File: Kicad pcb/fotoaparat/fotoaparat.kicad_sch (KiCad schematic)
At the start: 27 parts, among them J1 USB Konektor, J2 SWD, J3 LCD konektor, J5 Sd Karta, J6 UART, J7 Kamera, U1 STM32L496RETx, U2 Regulator 3.3v, U3 MCP73833-FCI/UN, Y1 HC49S-8-30-50-70-30-ATF

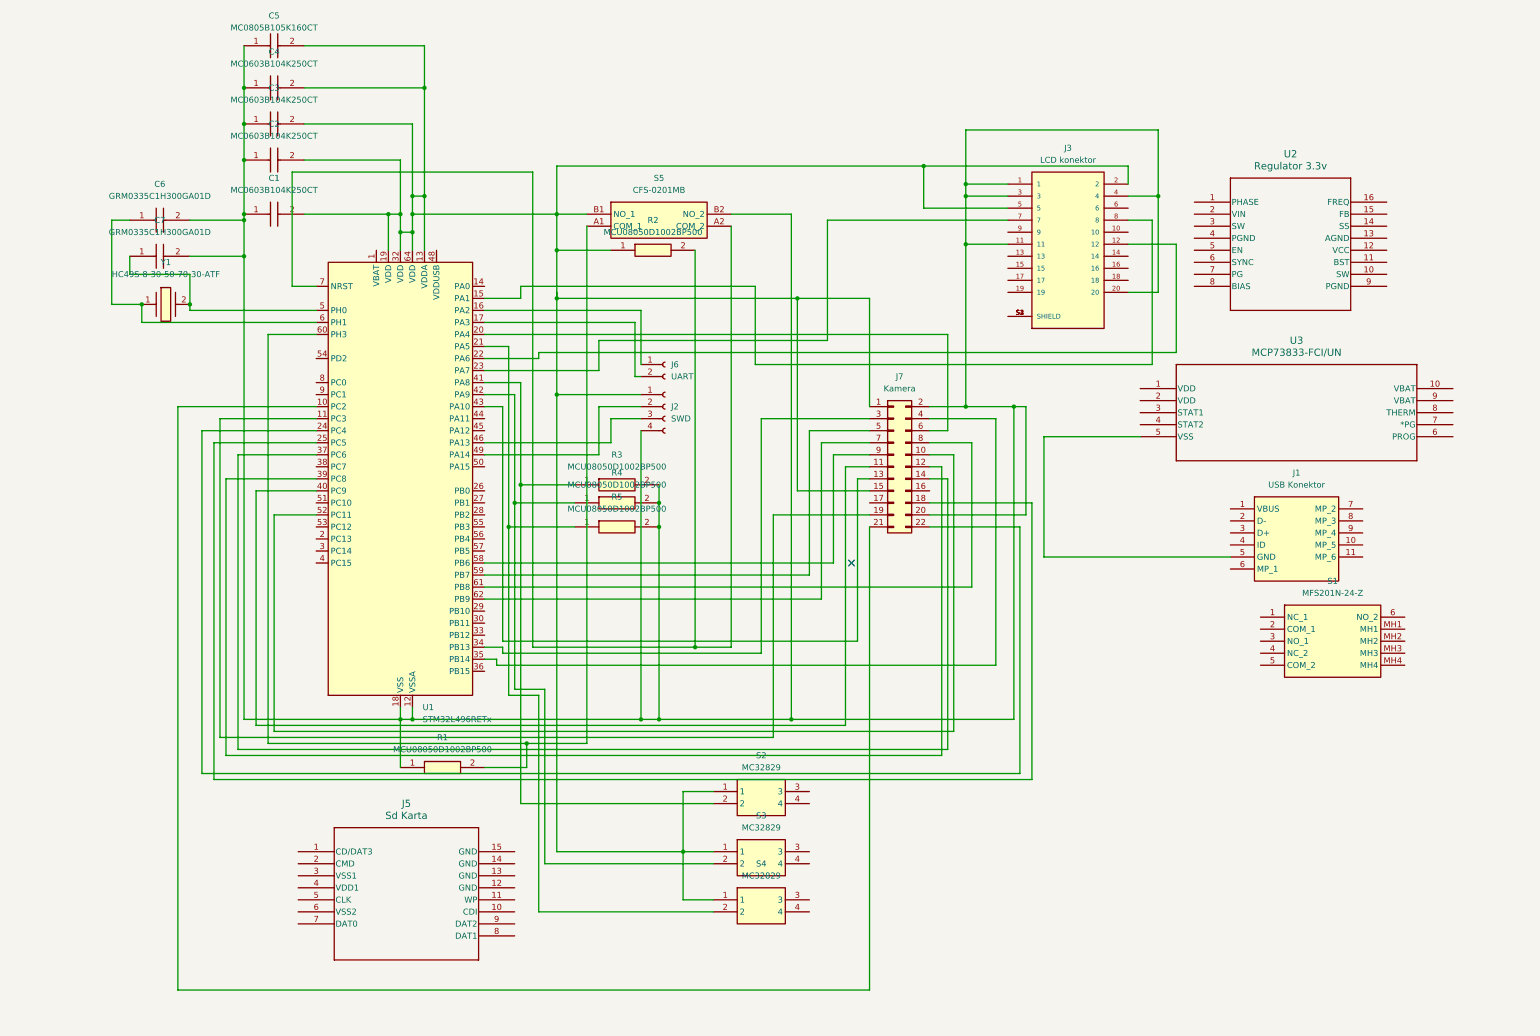
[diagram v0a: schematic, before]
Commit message: Baterie
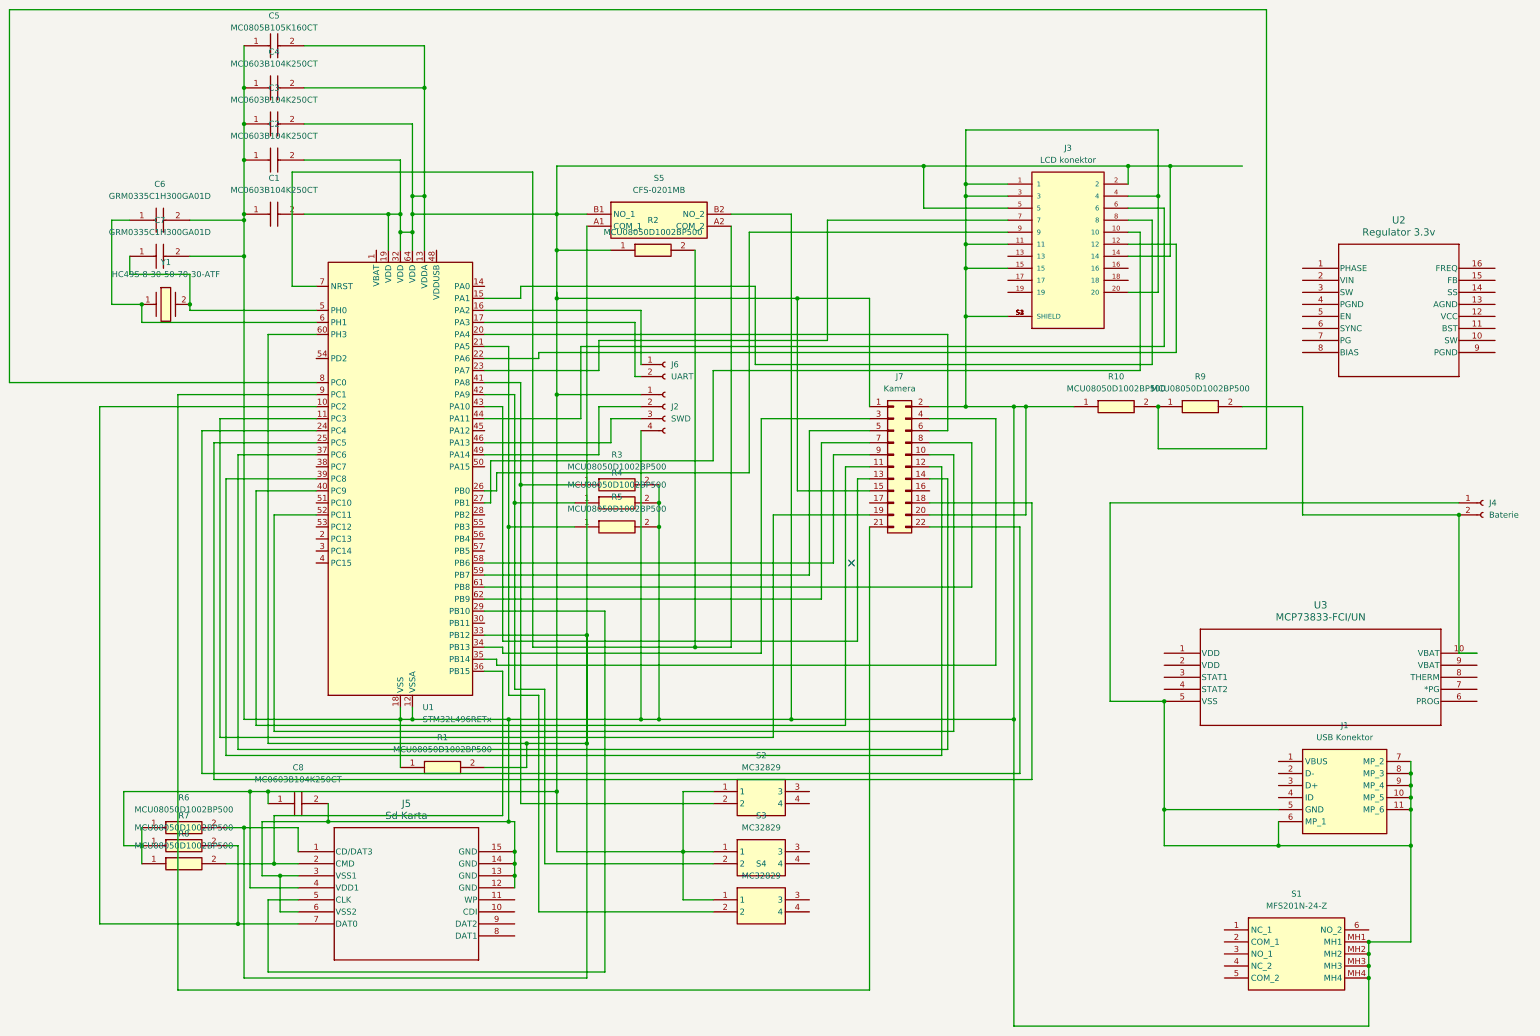
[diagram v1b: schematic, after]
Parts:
- added C8: MC0603B104K250CT, mc06:CAPC1608X87N, symbol MC0603B104K250CT:MC0603B104K250CT
- added J4: Baterie, symbol Connector:Conn_01x02_Socket
- added R10, R6, R7, R8, R9: MCU08050D1002BP500, 2012:RESC2012X55N, symbol MCU08050D1002BP500:MCU08050D1002BP500
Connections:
- net at S1.MH1: now also C1.1, C2.1, C3.1, C4.1, C5.1, C6.2, C7.2, J1.10 (MP_5), J1.11 (MP_6), J1.5 (GND), J1.6 (MP_1), J1.7 (MP_2), J1.8 (MP_3), J1.9 (MP_4), J2.4 (Pin_4), J3.1, J3.11, J3.15, J3.20, J3.3, J3.4, J3.S1 (SHIELD), J3.S2 (SHIELD), J3.S3 (SHIELD), J3.S4 (SHIELD), J5.12 (GND), J5.13 (GND), J5.14 (GND), J5.15 (GND), J5.3 (VSS1), J5.6 (VSS2), J7.2 (Pin_2), J7.20 (Pin_20), R1.1, R3.2, R4.2, R5.2, S1.MH2, S1.MH3, S1.MH4, S5.B2 (NO_2), U1.12 (VSSA), U1.18 (VSS), U1.31 (VSS), U1.47 (VSS), U1.63 (VSS), U3.5 (VSS), C8.2, J4.1 (Pin_1), R10.1
- net at C1.2, C2.2, C3.2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: now also J3.14, J5.4 (VDD1), C8.1, R6.1, R7.1, R8.1
- net at J7.21 (Pin_21): now also U1.9 (PC1); no longer U1.10 (PC2)
- net at U1.26 (PB0): now also J3.9
- net at U1.27 (PB1): now also J3.10
- net at U1.29 (PB10): now also J5.5 (CLK)
- net at U1.33 (PB12): now also J5.1 (CD/DAT3), R1.2, S5.A1 (COM_1), U1.60 (PH3), R6.2
- net at U1.36 (PB15): now also J5.2 (CMD), R8.2
- net at U1.44 (PA11): now also J3.6
- net at U1.8 (PC0): now also R10.2, R9.1
- net at J5.7 (DAT0): now also U1.10 (PC2), R7.2
- net at U3.10 (VBAT): now also J4.2 (Pin_2), R9.2
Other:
- moved on the sheet: J1, S1, U2, U3

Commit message: Přepojení součástek
vypadá to trochu lépe
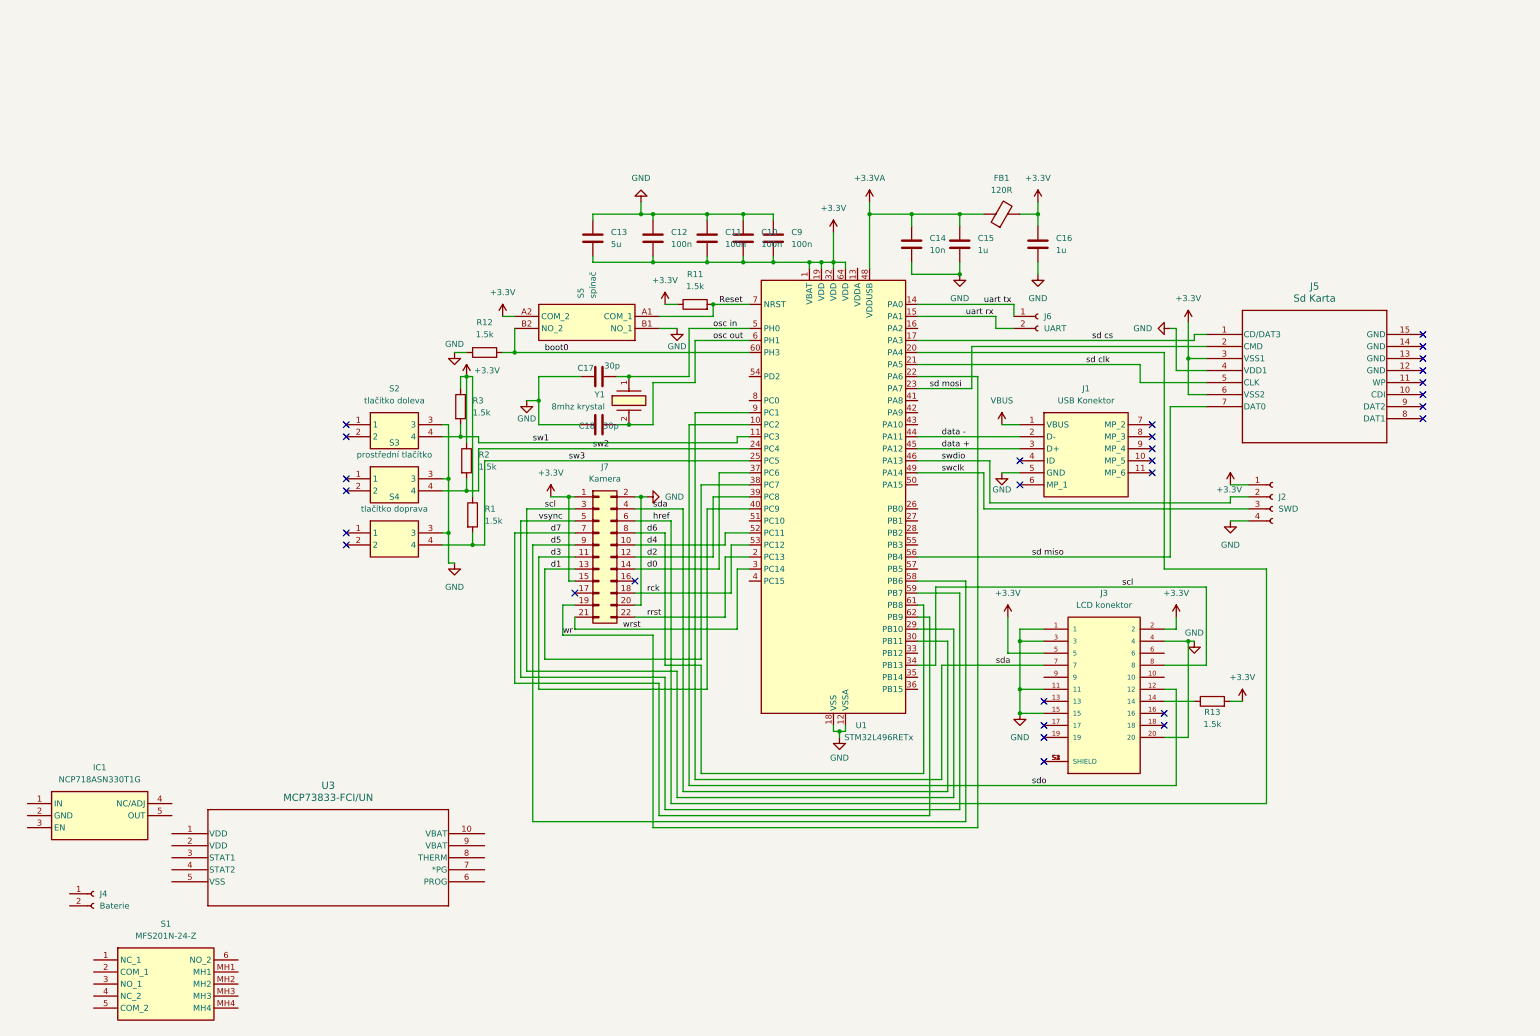
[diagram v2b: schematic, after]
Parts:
- removed C1, C2, C3, C4, C8: MC0603B104K250CT, mc06:CAPC1608X87N, symbol MC0603B104K250CT:MC0603B104K250CT
- removed C5: MC0805B105K160CT, mc08:CAPC2012X135N, symbol MC0805B105K160CT:MC0805B105K160CT
- removed C6, C7: GRM0335C1H300GA01D, grm033:GRM033D70J224ME01D, symbol GRM0335C1H300GA01D:GRM0335C1H300GA01D
- removed R1, R10, R2, R3, R4, R5, R6, R7, R8, R9: MCU08050D1002BP500, 2012:RESC2012X55N, symbol MCU08050D1002BP500:MCU08050D1002BP500
- removed U2: Regulator 3.3v, MPQ:QFN-3x4_MPQ4432_MNP, symbol 2025-09-30_17-10-32:MPQ4432GL-AEC1-P
- added C10, C11, C12, C9: 100n, Capacitor_SMD:C_0603_1608Metric_Pad1.08x0.95mm_HandSolder, symbol Device:C
- added C13: 5u, symbol Device:C
- added C14: 10n, Capacitor_SMD:C_0603_1608Metric_Pad1.08x0.95mm_HandSolder, symbol Device:C
- added C15, C16: 1u, symbol Device:C
- added C17, C18: 30p, Capacitor_SMD:C_0201_0603Metric_Pad0.64x0.40mm_HandSolder, symbol Device:C
- added FB1: 120R, symbol Device:FerriteBead
- added IC1: NCP718ASN330T1G, SOT95P280X100-5N, symbol NCP718ASN330T1G:NCP718ASN330T1G
- added R1, R11, R12, R13, R2, R3: 1.5k, symbol Device:R
- S2: value MC32829 -> tlačítko doleva
- S3: value MC32829 -> prostřední tlačítko
- S4: value MC32829 -> tlačítko doprava
- S5: value CFS-0201MB -> spínač
- Y1: value HC49S-8-30-50-70-30-ATF -> 8mhz krystal
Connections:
- net at J4.2 (Pin_2): no longer U3.10 (VBAT)
- net +3.3V: now reaches J2.1 (Pin_1), J3.2, J3.5, J7.1 (Pin_1), J7.15 (Pin_15), U1.19 (VDD), U1.32 (VDD), U1.64 (VDD)
- net +3.3V: now also J5.3 (VSS1), J5.6 (VSS2), S5.A2 (COM_2), U1.1 (VBAT), C10.2, C11.2, C12.2, C13.2, C16.1, C9.2, FB1.2, R1.1, R11.1, R13.2, R2.1, R3.1; no longer J3.14, J5.4 (VDD1), S2.1, S3.1, S4.1, S5.B1 (NO_1), U1.13 (VDDA)
- net d4: now reaches J7.10 (Pin_10), U1.52 (PC11)
- net d3: now reaches J7.11 (Pin_11), U1.40 (PC9)
- net d2: now reaches J7.12 (Pin_12), U1.39 (PC8)
- net at U1.43 (PA10): no longer J7.13 (Pin_13)
- net d0: now reaches J7.14 (Pin_14), U1.37 (PC6)
- net rck: now reaches J7.18 (Pin_18)
- net rck: now also U1.53 (PC12); no longer U1.25 (PC5)
- net sw1: now reaches U1.11 (PC3)
- net sw1: now also S2.4, R3.2; no longer J7.19 (Pin_19)
- net sda: now reaches U1.9 (PC1)
- net sda: now also J3.7, J7.4 (Pin_4), U1.30 (PB11); no longer J7.21 (Pin_21)
- net rrst: now reaches J7.22 (Pin_22)
- net rrst: now also U1.2 (PC13); no longer U1.24 (PC4)
- net scl: now reaches J7.3 (Pin_3), U1.34 (PB13)
- net scl: now also J3.8, U1.29 (PB10)
- net at U1.35 (PB14): no longer J7.4 (Pin_4)
- net vsync: now reaches J7.5 (Pin_5), U1.59 (PB7)
- net href: now reaches J7.6 (Pin_6), U1.20 (PA4)
- net d7: now reaches J7.7 (Pin_7), U1.62 (PB9)
- net d6: now reaches J7.8 (Pin_8), U1.61 (PB8)
- net d5: now reaches J7.9 (Pin_9), U1.58 (PB6)
- net sd miso: now reaches J5.7 (DAT0)
- net sd miso: now also U1.56 (PB4); no longer U1.10 (PC2)
- net uart tx: now reaches U1.14 (PA0)
- net uart tx: now also J6.1 (Pin_1)
- net uart rx: now reaches U1.15 (PA1)
- net uart rx: now also J6.2 (Pin_2); no longer J3.8
- net at U1.16 (PA2): no longer J6.1 (Pin_1)
- net sd cs: now reaches U1.17 (PA3)
- net sd cs: now also J5.1 (CD/DAT3); no longer J6.2 (Pin_2)
- net at S4.2: no longer U1.21 (PA5)
- net sdo: now reaches J3.12
- net sdo: now also U1.10 (PC2); no longer U1.22 (PA6)
- net sd mosi: now reaches U1.23 (PA7)
- net sd mosi: now also J5.2 (CMD); no longer J3.7
- net at U1.26 (PB0): no longer J3.9
- net at U1.27 (PB1): no longer J3.10
- net sd clk: now reaches J5.5 (CLK)
- net sd clk: now also U1.21 (PA5); no longer U1.29 (PB10)
- net wrst: now reaches U1.3 (PC14)
- net wrst: now also J7.21 (Pin_21)
- net at U1.36 (PB15): no longer J5.2 (CMD)
- net d1: now reaches U1.38 (PC7)
- net d1: now also J7.13 (Pin_13)
- net at U1.41 (PA8): no longer S2.2
- net at U1.42 (PA9): no longer S3.2
- net at J3.6: no longer U1.44 (PA11)
- net data +: now reaches U1.45 (PA12)
- net data +: now also J1.3 (D+)
- net swclk: now reaches J2.3 (Pin_3)
- net swclk: now also U1.49 (PA14); no longer U1.46 (PA13)
- net +3.3VA: now reaches U1.48 (VDDUSB)
- net +3.3VA: now also C14.1, C15.1, FB1.1
- net swdio: now reaches J2.2 (Pin_2)
- net swdio: now also U1.46 (PA13); no longer U1.49 (PA14)
- net osc in: now reaches U1.5 (PH0)
- net osc in: now also Y1.1, C17.2; no longer Y1.2
- net osc out: now reaches U1.6 (PH1)
- net osc out: now also Y1.2, C18.2; no longer Y1.1
- net Reset: now reaches U1.7 (NRST)
- net Reset: now also S5.A1 (COM_1), R11.2; no longer S5.A2 (COM_2)
- net GND: now reaches S4.3
- net GND: now also J1.5 (GND), J2.4 (Pin_4), J3.1, J3.11, J3.15, J3.20, J3.3, J3.4, J5.4 (VDD1), J7.2 (Pin_2), J7.20 (Pin_20), S2.3, S3.3, S5.B1 (NO_1), U1.12 (VSSA), U1.18 (VSS), U1.31 (VSS), U1.47 (VSS), U1.63 (VSS), C10.1, C11.1, C12.1, C13.1, C14.2, C15.2, C16.2, C17.1, C18.1, C9.1, R12.1
- net sw3: now reaches S4.4
- net sw3: now also U1.25 (PC5), R1.2
- net sw2: now reaches S3.4
- net sw2: now also U1.24 (PC4), R2.2
- net VBUS: now reaches J1.1 (VBUS)
- net data -: now reaches J1.2 (D-)
- net data -: now also U1.44 (PA11)
- new net: J3.14, R13.1
- new net: J3.S1 (SHIELD), J3.S2 (SHIELD), J3.S3 (SHIELD), J3.S4 (SHIELD)
- new net boot0: R12.2, S5.B2 (NO_2), U1.60 (PH3)
- new net wr: J7.19 (Pin_19), U1.22 (PA6)
- now unconnected: J1.10 (MP_5), J1.11 (MP_6), J1.6 (MP_1), J1.7 (MP_2), J1.8 (MP_3), J1.9 (MP_4), J4.1 (Pin_1), J5.12 (GND), J5.13 (GND), J5.14 (GND), J5.15 (GND), S1.MH1, S1.MH2, S1.MH3, S1.MH4, U1.33 (PB12), U3.5 (VSS)
- no-connect marks 1 -> 29
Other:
- moved on the sheet: J1, J2, J3, J4, J5, J6, J7, S1, S2, S3, S4, S5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

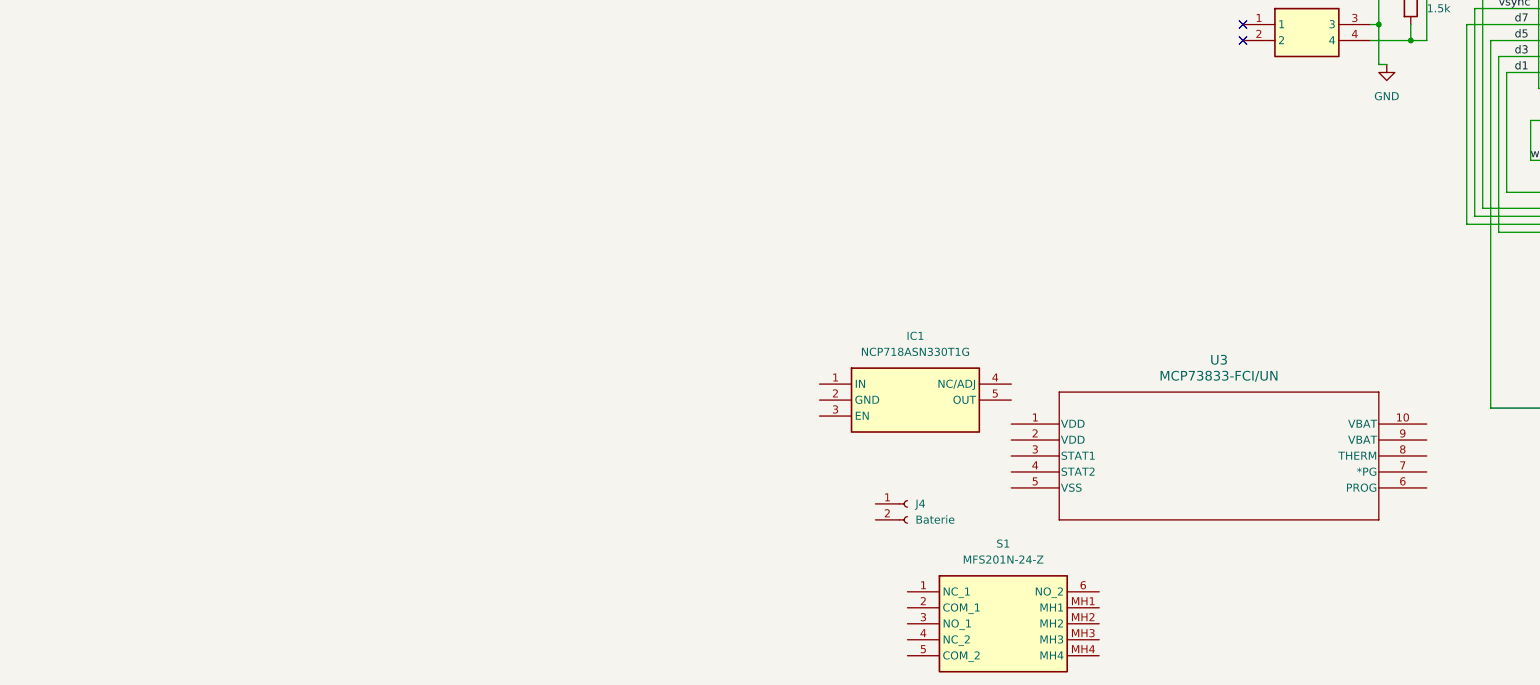
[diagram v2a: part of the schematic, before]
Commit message: Baterie nabíječka
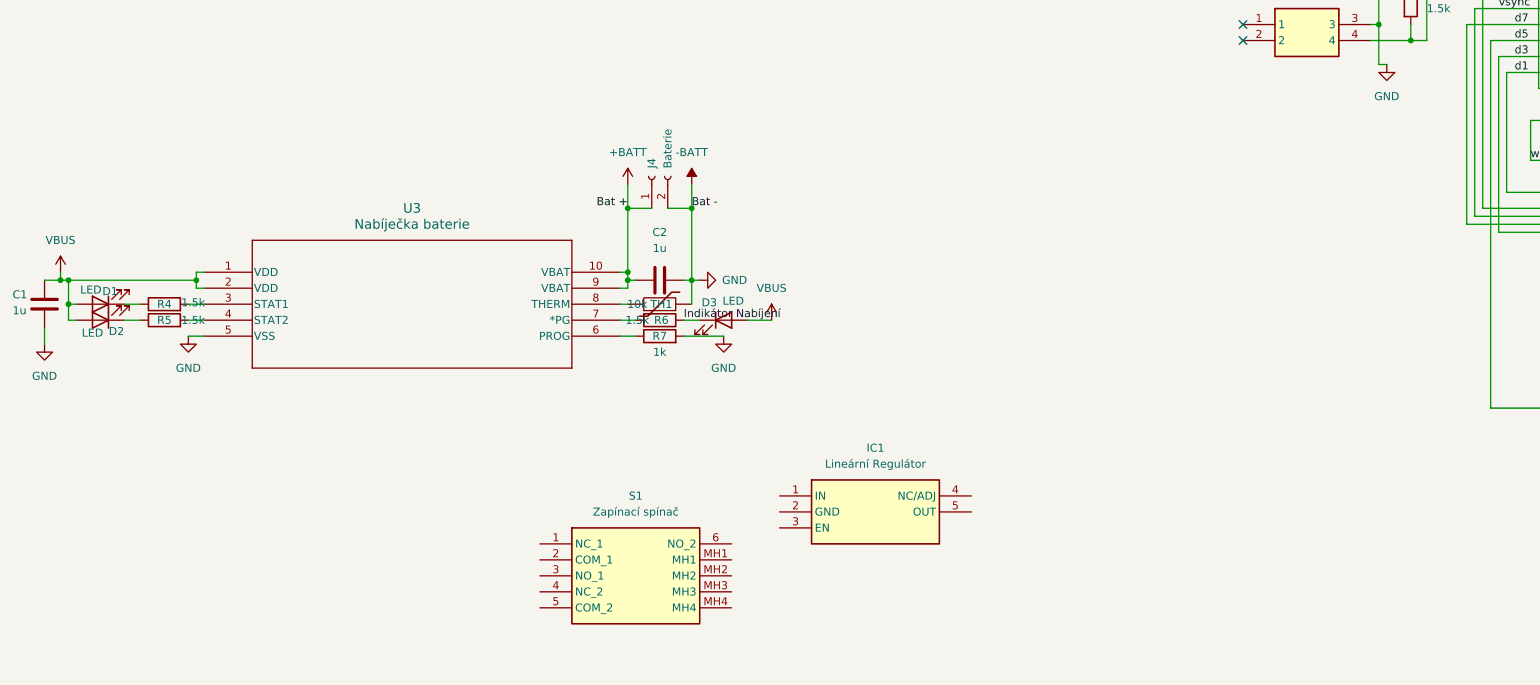
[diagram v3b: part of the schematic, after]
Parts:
- added C1, C2: 1u, symbol Device:C
- added D1, D2, D3: LED, symbol Device:LED
- added R4, R5, R6: 1.5k, symbol Device:R
- added R7: 1k, symbol Device:R
- added TH1: 10k, symbol Device:Thermistor
- IC1: value NCP718ASN330T1G -> Lineární Regulátor
- S1: value MFS201N-24-Z -> Zapínací spínač
- U3: value MCP73833-FCI/UN -> Nabíječka baterie
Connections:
- net GND is gone; now on net -BATT: C10.1, C11.1, C12.1, C13.1, C14.2, C15.2, C16.2, C17.1, C18.1, C9.1, J1.5 (GND), J2.4 (Pin_4), J3.1, J3.11, J3.15, J3.20, J3.3, J3.4, J5.4 (VDD1), J7.2 (Pin_2), J7.20 (Pin_20), R12.1, S2.3, S3.3, S4.3, S5.B1 (NO_1), U1.12 (VSSA), U1.18 (VSS), U1.31 (VSS), U1.47 (VSS), U1.63 (VSS)
- net VBUS: now also U3.1 (VDD), U3.2 (VDD), C1.1, D1.2 (A), D2.2 (A), D3.2 (A)
- net +BATT: now reaches J4.1 (Pin_1)
- net +BATT: now also U3.10 (VBAT), U3.9 (VBAT), C2.1
- net -BATT: now reaches J4.2 (Pin_2)
- net -BATT: now also U3.5 (VSS), C1.2, C2.2, R7.2, TH1.2
- net at U3.3 (STAT1): now also R4.2
- net at U3.4 (STAT2): now also R5.2
- net at U3.6 (PROG): now also R7.1
- net at U3.7 (*PG): now also R6.2
- net at U3.8 (THERM): now also TH1.1
- new net: D2.1 (K), R5.1
- new net: D1.1 (K), R4.1
- new net Indikátor Nabíjení: D3.1 (K), R6.1
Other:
- moved on the sheet: IC1, J4, S1, U3
